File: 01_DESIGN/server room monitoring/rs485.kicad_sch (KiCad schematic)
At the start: 0 parts

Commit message: Update project files
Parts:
- added C9: 0.1uF, symbol Device:C
- added D4: SM712_SOT23, Package_TO_SOT_SMD:SOT-23, symbol Diode:SM712_SOT23
- added J3: Screw_Terminal_01x03, symbol Connector:Screw_Terminal_01x03
- added J4: Header 2x1, Connector_PinHeader_1.00mm:PinHeader_1x02_P1.00mm_Vertical, symbol AL:Header 2x1
- added R5: 10k, symbol Device:R
- added R7, R9: 4.7k, symbol Device:R
- added R8: 120R, symbol Device:R
- added U4: SP3485EN, Package_SO:SOIC-8_3.9x4.9mm_P1.27mm, symbol Interface_UART:SP3485EN
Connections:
- new net: D4.1 (A1), J3.1 (Pin_1), J4.1, R7.2, R8.1, U4.6 (A)
- new net: D4.2 (A2), J3.2 (Pin_2), J4.2, R8.2, R9.1, U4.7 (B)
- new net: C9.2, U4.8 (VCC)
- new net +3.3V: C9.1, R7.1
- new net GND: D4.3 (common), J3.3 (Pin_3), R5.1, R9.2, U4.5 (GND)
- new net RS485_DE_~{RE}: R5.2, U4.2 (~{RE}), U4.3 (DE)
- new net RS485_RX: U4.1 (RO)
- new net RS485_TX: U4.4 (DI)

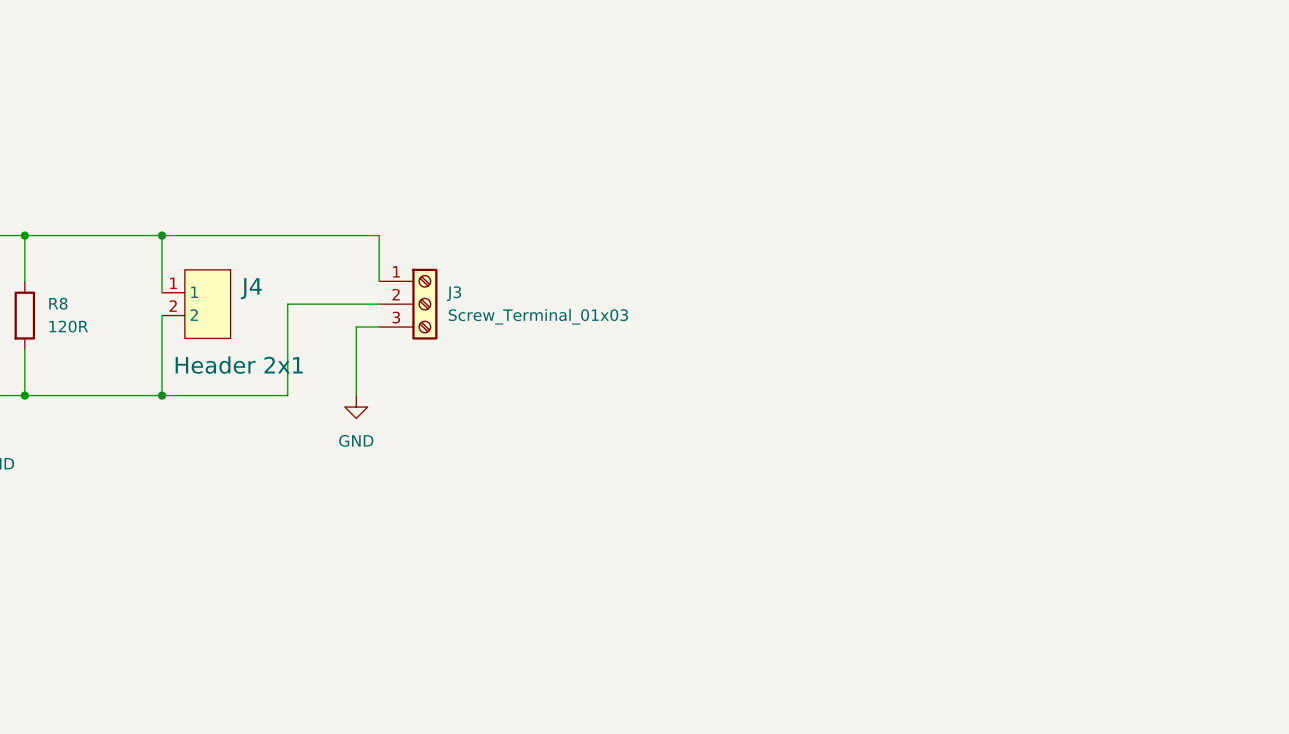
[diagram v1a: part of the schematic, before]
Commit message: Update project files
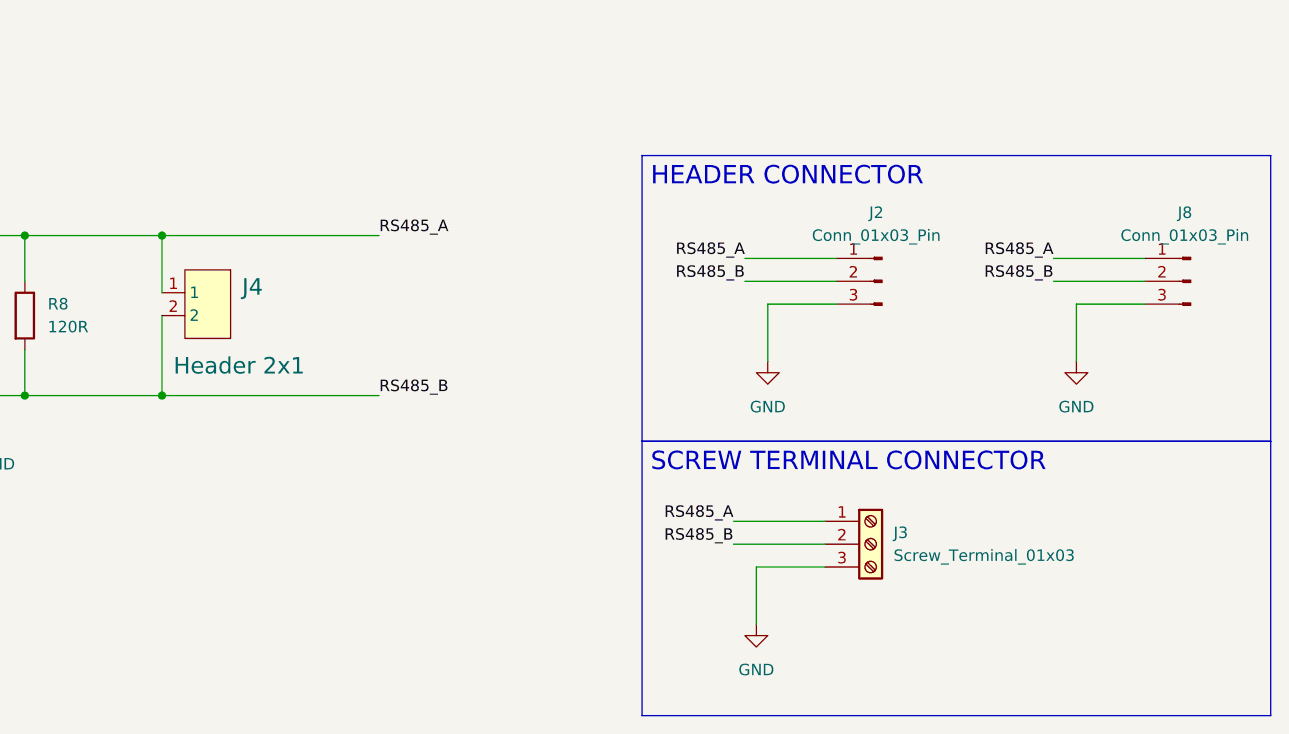
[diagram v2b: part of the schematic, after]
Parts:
- added J2, J8: Conn_01x03_Pin, Connector:FanPinHeader_1x03_P2.54mm_Vertical, symbol Connector:Conn_01x03_Pin
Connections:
- net GND: now also J2.3 (Pin_3), J8.3 (Pin_3)
- net RS485_A: now reaches D4.1 (A1), J3.1 (Pin_1), J4.1, R7.2, R8.1, U4.6 (A)
- net RS485_A: now also J2.1 (Pin_1), J8.1 (Pin_1)
- net RS485_B: now reaches D4.2 (A2), J3.2 (Pin_2), J4.2, R8.2, R9.1, U4.7 (B)
- net RS485_B: now also J2.2 (Pin_2), J8.2 (Pin_2)
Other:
- moved on the sheet: J3

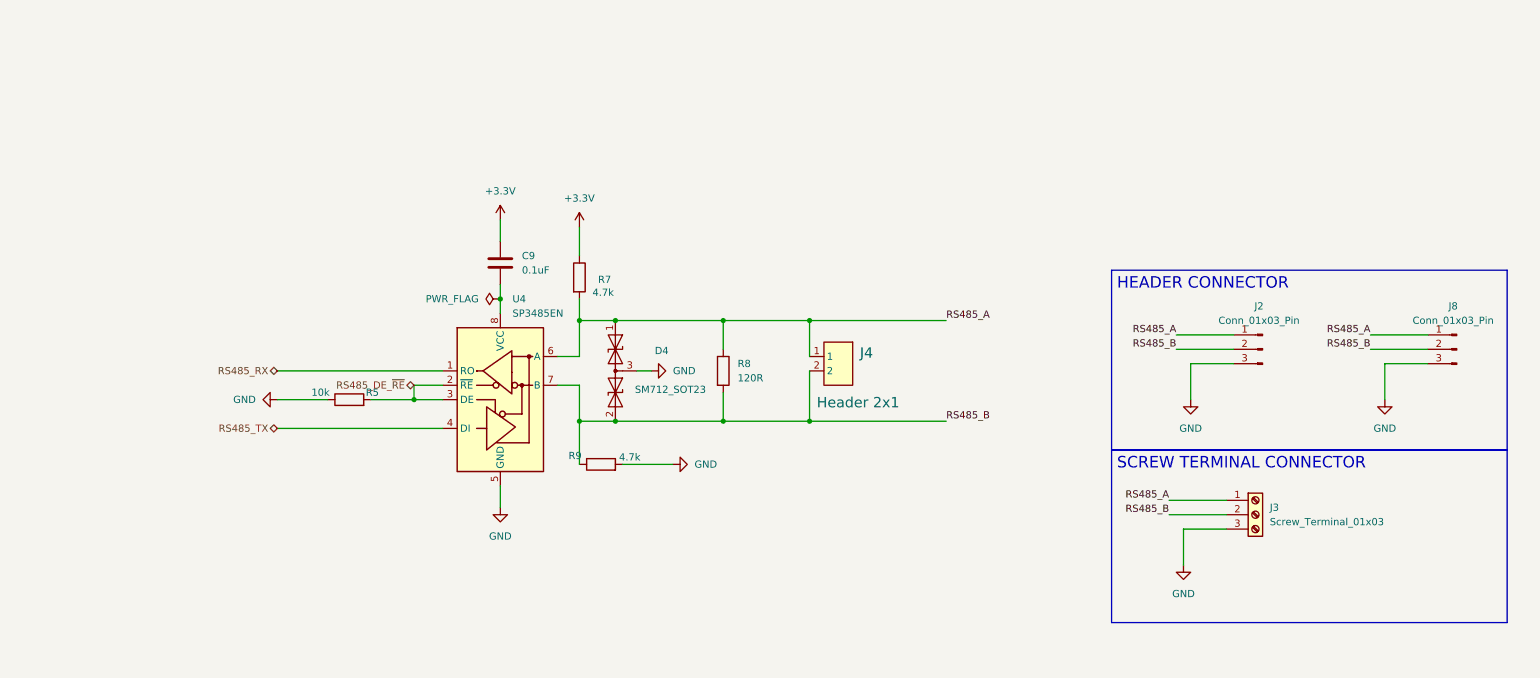
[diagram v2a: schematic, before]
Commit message: Update project files
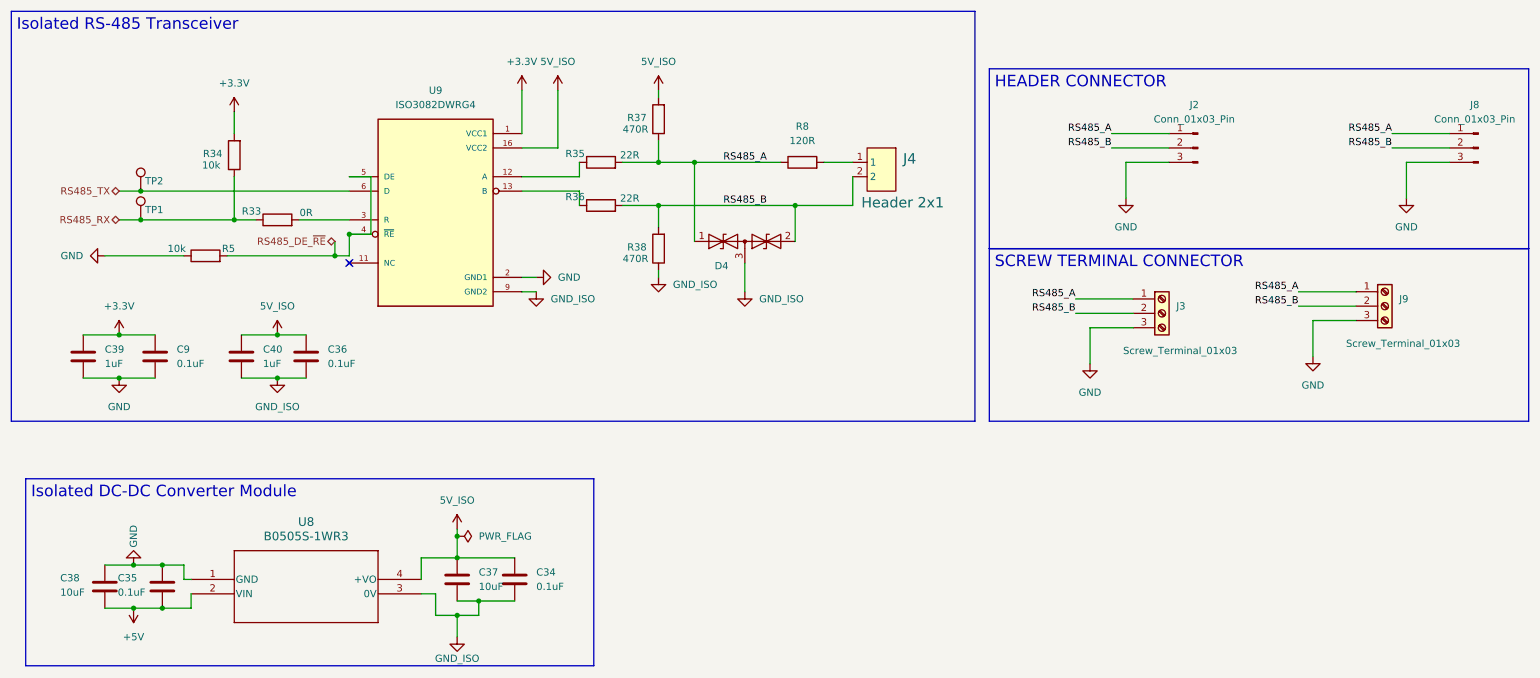
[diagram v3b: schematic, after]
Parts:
- removed R7, R9: 4.7k, symbol Device:R
- removed U4: SP3485EN, Package_SO:SOIC-8_3.9x4.9mm_P1.27mm, symbol Interface_UART:SP3485EN
- added C34, C35, C36: 0.1uF, Capacitor_SMD:C_0805_2012Metric, symbol Device:C
- added C37, C38: 10uF, Capacitor_SMD:C_0805_2012Metric, symbol Device:C
- added C39, C40: 1uF, Capacitor_SMD:C_0805_2012Metric, symbol Device:C
- added J9: Screw_Terminal_01x03, TerminalBlock_CUI:TerminalBlock_CUI_TB007-508-03_1x03_P5.08mm_Horizontal, symbol Connector:Screw_Terminal_01x03
- added R33: 0R, Resistor_SMD:R_0805_2012Metric, symbol Device:R
- added R34: 10k, Resistor_SMD:R_0805_2012Metric, symbol Device:R
- added R35, R36: 22R, Resistor_SMD:R_0805_2012Metric, symbol Device:R
- added R37, R38: 470R, Resistor_SMD:R_0805_2012Metric, symbol Device:R
- added TP1, TP2: TestPoint, TestPoint:TestPoint_Pad_D1.0mm, symbol Connector:TestPoint
- added U8: B0505S-1WR3, footprints:SIP4_B_S-1WR3_MNS, symbol 2026-10-18_17-37-38:B0505S-1WR3
- added U9: ISO3082DWRG4, ISO3082DWRG4:SOIC127P1030X265-16N, symbol ISO3082DWRG4:ISO3082DWRG4
- C9: footprint (none) -> Capacitor_SMD:C_0805_2012Metric
- J3: footprint (none) -> TerminalBlock_CUI:TerminalBlock_CUI_TB007-508-03_1x03_P5.08mm_Horizontal
- R5, R8: footprint (none) -> Resistor_SMD:R_0805_2012Metric
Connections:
- net +3.3V: now also C39.1, R34.2, U9.1 (VCC1)
- net GND: now also C9.2, C35.1, C38.1, C39.2, J9.3 (Pin_3), U8.1 (GND), U9.2 (GND1), U9.7 (GND1), U9.8 (GND1); no longer D4.3 (common)
- net RS485_A: now also J9.1 (Pin_1), R35.2, R37.1; no longer J4.1
- net RS485_B: now also J9.2 (Pin_2), R36.2, R38.2; no longer R8.2
- net RS485_DE_~{RE}: now also U9.4 (~{RE}), U9.5 (DE)
- net RS485_RX: now also R33.1, R34.1, TP1.1
- net RS485_TX: now also TP2.1, U9.6 (D)
- new net: J4.1, R8.2
- new net: R33.2, U9.3 (R)
- new net: R35.1, U9.12 (A)
- new net: U9.11 (NC), U9.14 (NC)
- new net: R36.1, U9.13 (B)
- new net +5V: C35.2, C38.2, U8.2 (VIN)
- new net 5V_ISO: C34.1, C36.1, C37.1, C40.1, R37.2, U8.4 (+VO), U9.16 (VCC2)
- new net GND2: C34.2, C36.2, C37.2, C40.2, D4.3 (common), R38.1, U8.3 (0V), U9.10 (GND2), U9.15 (GND2), U9.9 (GND2)
- no-connect marks 0 -> 1
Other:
- moved on the sheet: C9, D4, J2, J3, J4, J8, R5, R8
